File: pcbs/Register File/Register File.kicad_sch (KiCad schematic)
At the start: 1 part, among them J101 Conn_02x20_Odd_Even

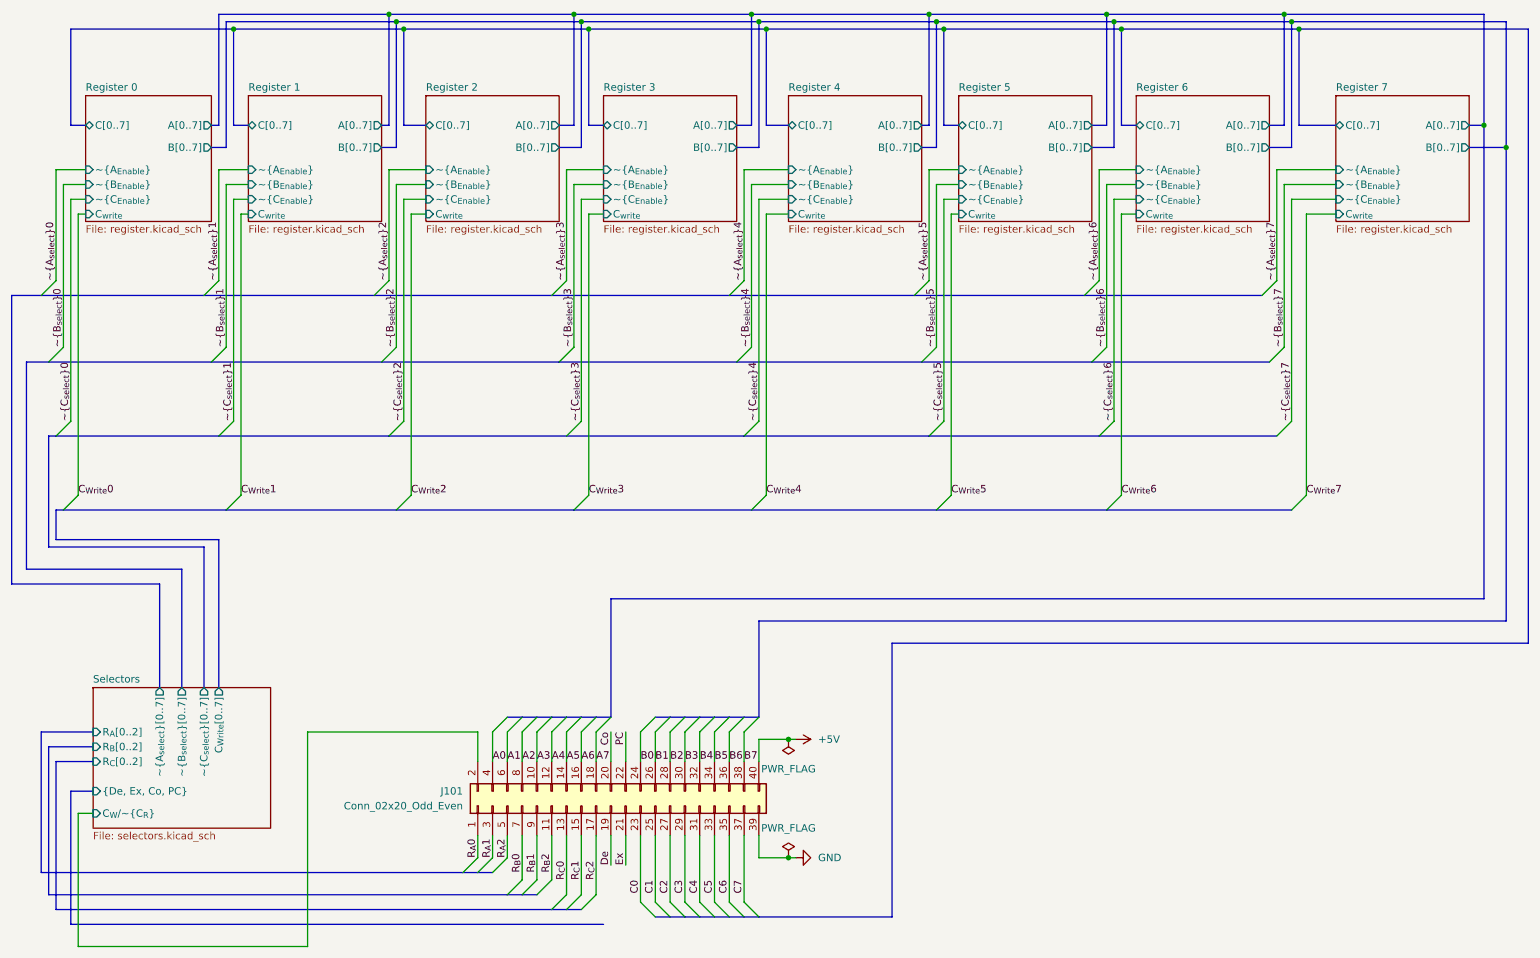
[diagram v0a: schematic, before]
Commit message: Lots of rethinking
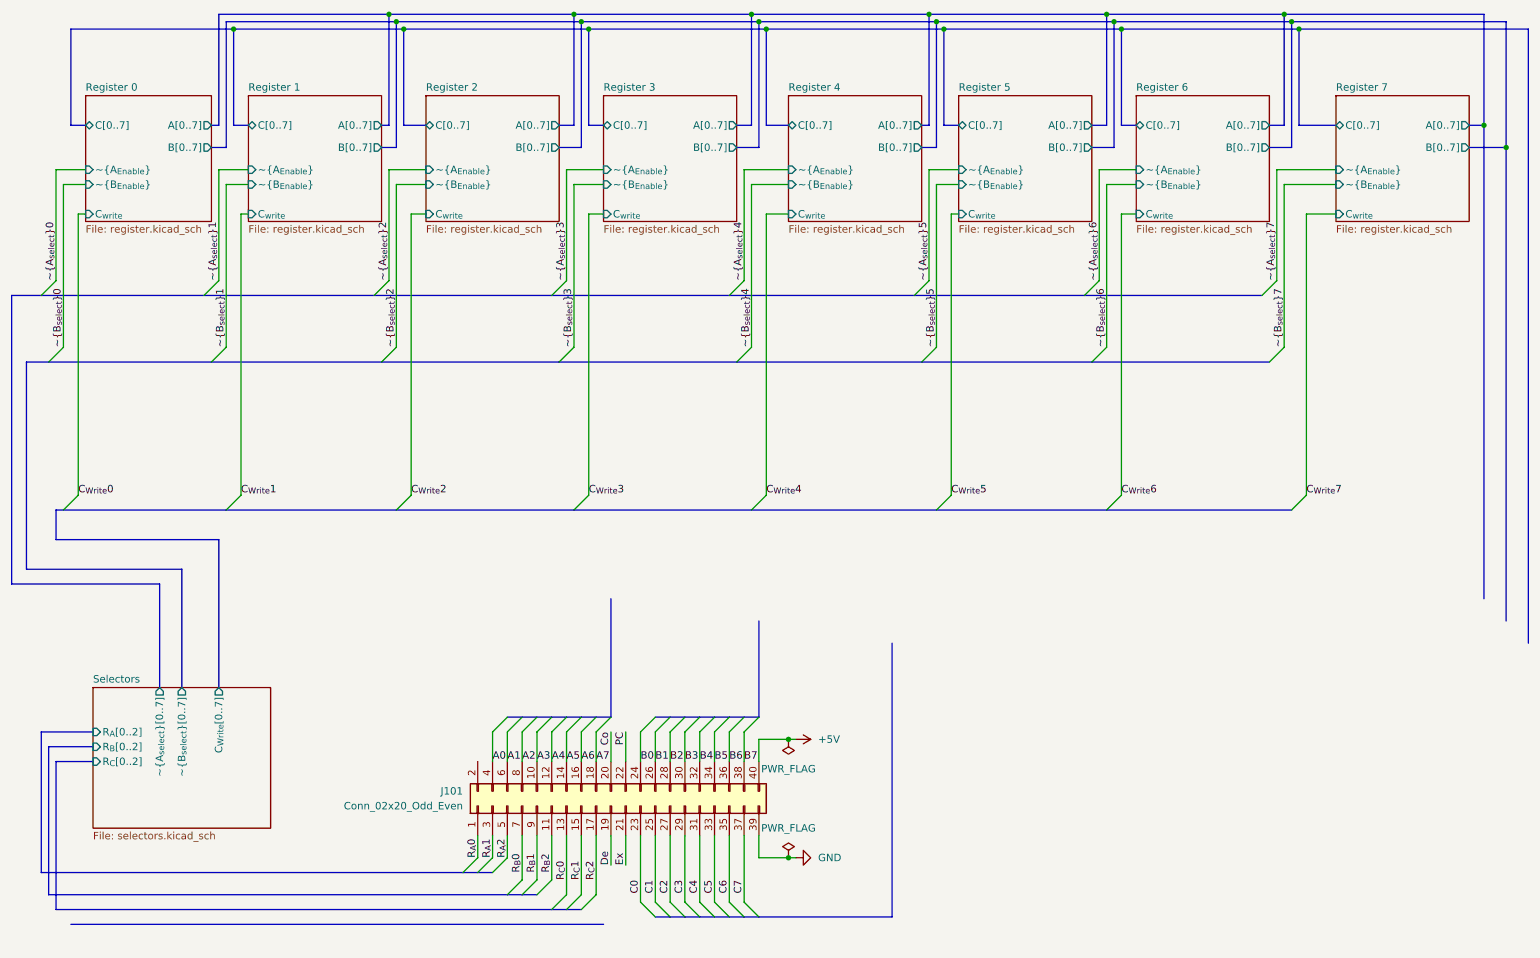
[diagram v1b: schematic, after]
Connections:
- net Selectors/C_{W}/~{C_{R}}: no longer names the net of J101.2 (Pin_2)
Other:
- sheet Register 0 ports: added none; removed ~{C_{Enable}}
- sheet Register 1 ports: added none; removed ~{C_{Enable}}
- sheet Register 2 ports: added none; removed ~{C_{Enable}}
- sheet Register 3 ports: added none; removed ~{C_{Enable}}
- sheet Register 4 ports: added none; removed ~{C_{Enable}}
- sheet Register 5 ports: added none; removed ~{C_{Enable}}
- sheet Register 6 ports: added none; removed ~{C_{Enable}}
- sheet Register 7 ports: added none; removed ~{C_{Enable}}
- sheet Selectors ports: added none; removed C_{W}/~{C_{R}}, {De, Ex, Co, PC}, ~{C_{select}}[0..7]
